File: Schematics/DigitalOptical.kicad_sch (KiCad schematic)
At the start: 112 parts, among them Q1 BSS138, Q2 BSS138, Q3 BSS138, Q4 BSS138, Q5 BSS138, Q6 BSS138, U100 PC817, U63 PC817, U64 PC817, U65 PCF8575, U66 PC817, U67 PC817, U68 PC817, U69 PC817, U70 PC817, U71 PC817, U72 PC817, U73 PC817, U74 LM1117-3.3, U75 PC817, U76 PC817, U77 PCF8575, U78 PCF8575, U79 PC817, U80 PC817, U81 PC817, U82 PC817, U83 PC817, U84 PC817, U85 PC817, U86 PC817, U87 LM1117-3.3, U88 LM1117-3.3, U89 PC817, U90 PC817, U91 PC817, U92 PC817, U93 PC817, U94 PC817, U95 PC817, U96 PC817, U97 PC817, U98 PC817, U99 PC817

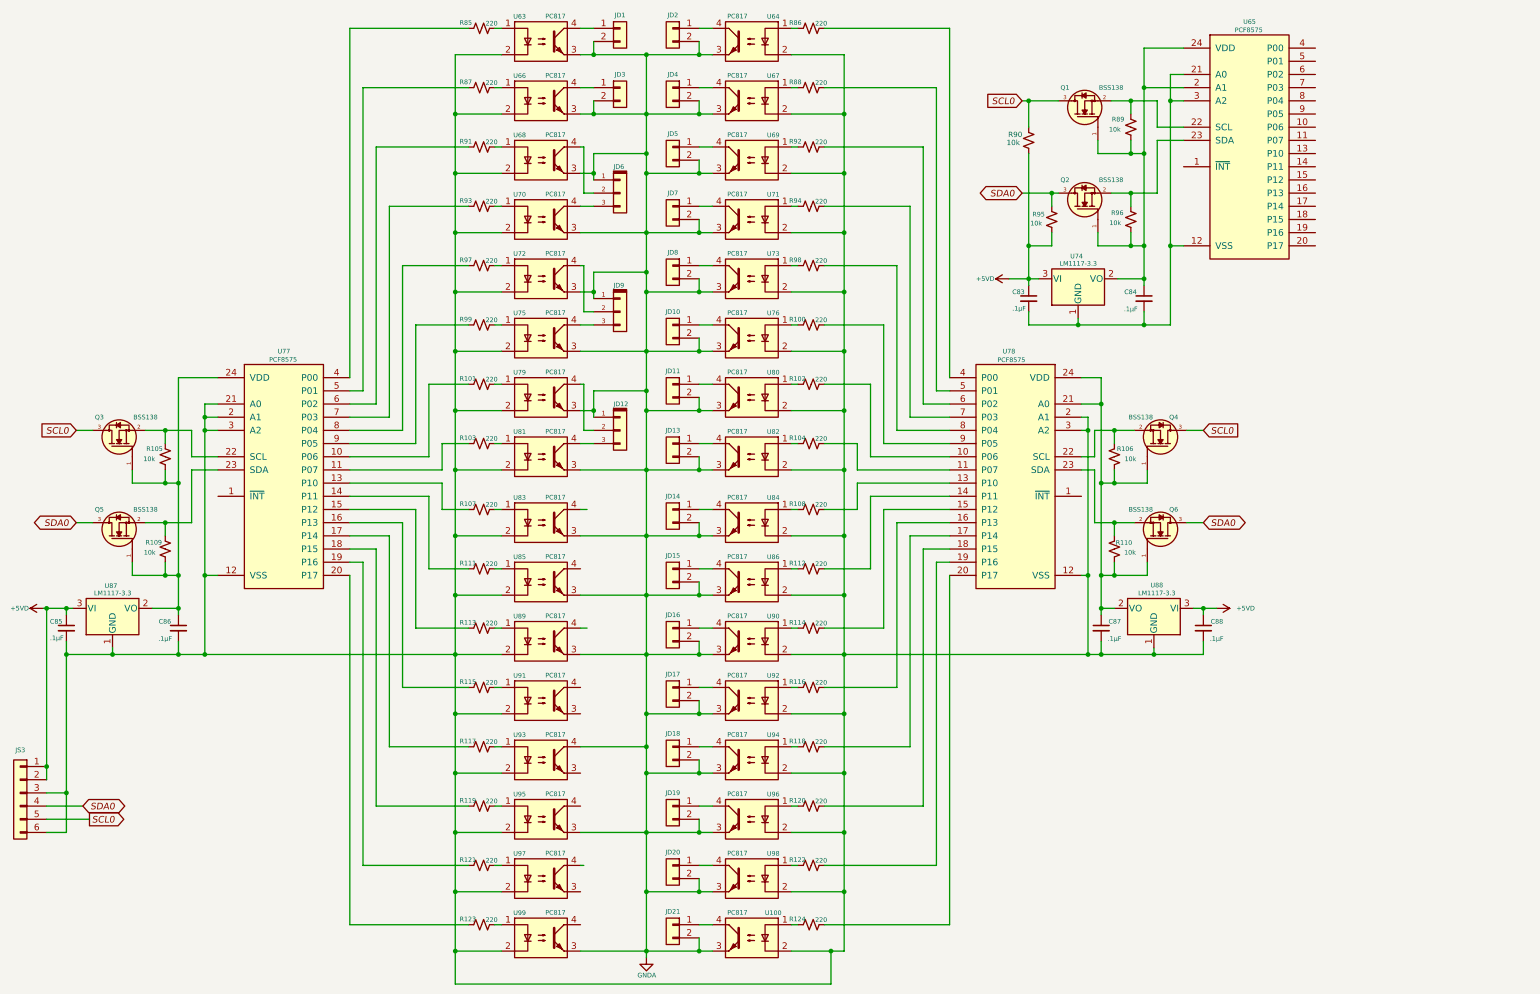
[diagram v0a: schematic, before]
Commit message: Prelude to split configurations.
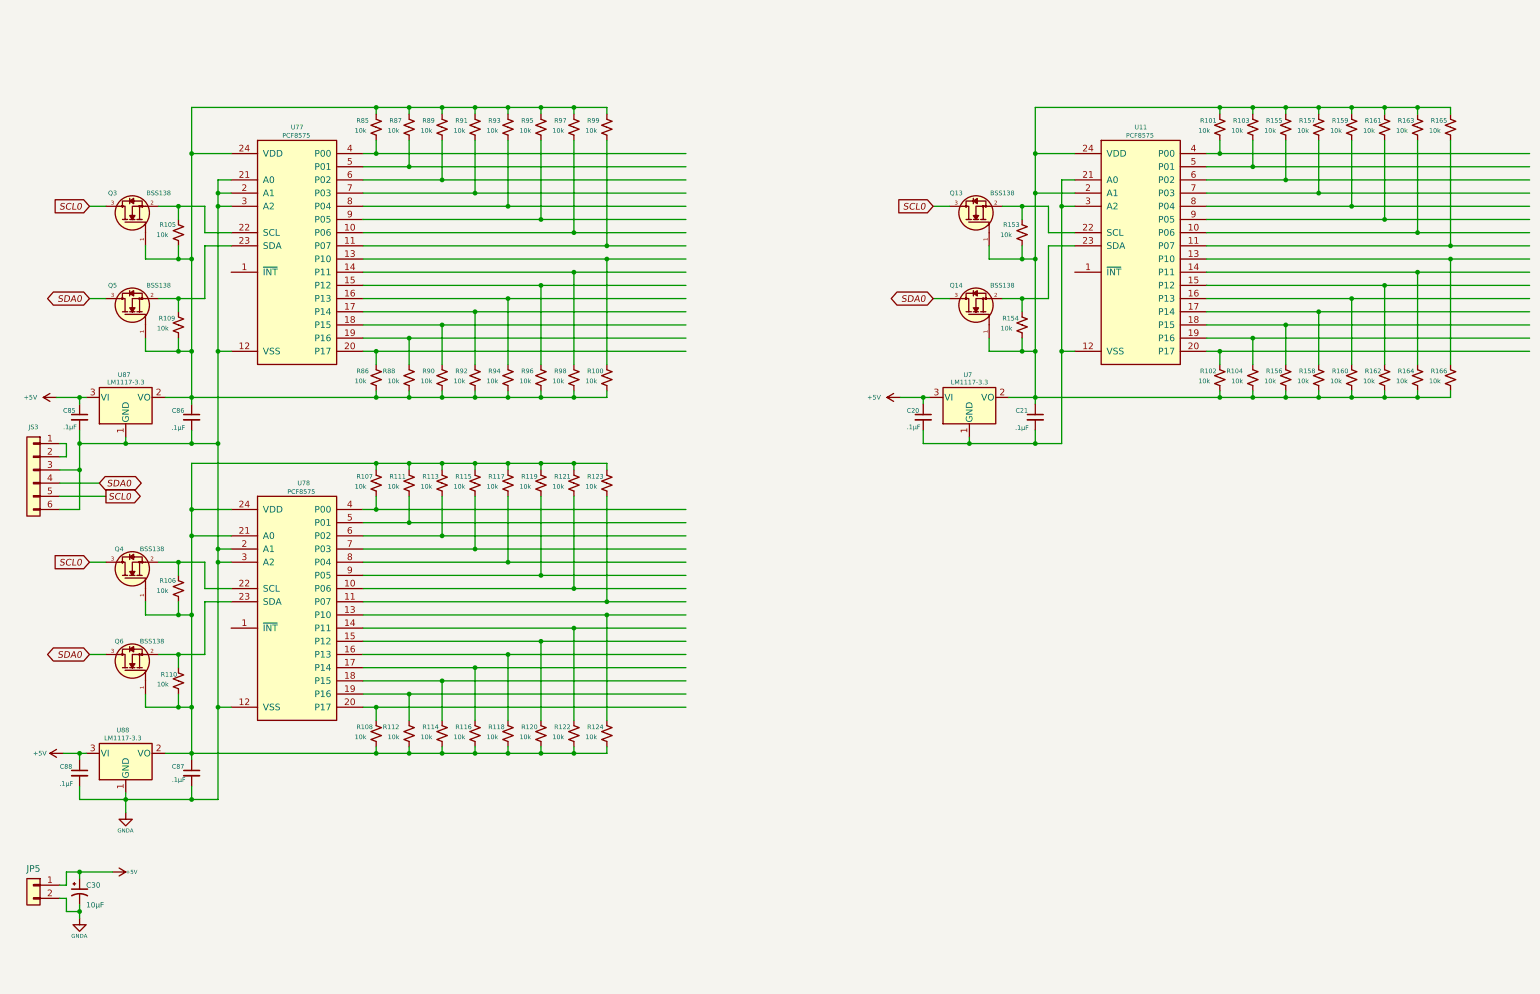
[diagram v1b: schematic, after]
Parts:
- removed C83, C84: .1µF, symbol Device:C_Small
- removed JD1, JD10, JD11, JD13, JD14, JD15, JD16, JD17, JD18, JD19, JD2, JD20, JD21, JD3, JD4, JD5, JD7, JD8: From 12v Analog, symbol Connector_Generic:Conn_01x02
- removed JD12, JD6, JD9: Conn_01x03, symbol Connector_keyed_kicad_sym:Conn_01x03
- removed Q1, Q2: BSS138, digikey-footprints:SOT-23-3, symbol dk_Transistors-FETs-MOSFETs-Single:BSS138
- removed U100, U63, U64, U66, U67, U68, U69, U70, U71, U72, U73, U75, U76, U79, U80, U81, U82, U83, U84, U85, U86, U89, U90, U91, U92, U93, U94, U95, U96, U97, U98, U99: PC817, Package_DIP:DIP-4_W7.62mm, symbol Isolator:PC817
- removed U65: PCF8575, IPC7351-Nominal:SOP65P775X200-24, symbol NXP:PCF8575
- removed U74: LM1117-3.3, symbol Regulator_Linear:LM1117-3.3
- added C20, C21: .1µF, symbol Device:C_Small
- added C30: 10µF, symbol Device:C_Polarized_Small_US
- added JP5: From 12v Analog, symbol Connector_Generic:Conn_01x02
- added Q13, Q14: BSS138, digikey-footprints:SOT-23-3, symbol dk_Transistors-FETs-MOSFETs-Single:BSS138
- added R153, R154, R155, R156, R157, R158, R159, R160, R161, R162, R163, R164, R165, R166: 10k, symbol Device:R_Small_US
- added U11: PCF8575, IPC7351-Nominal:SOP65P775X200-24, symbol NXP:PCF8575
- added U7: LM1117-3.3, symbol Regulator_Linear:LM1117-3.3
- R100, R101, R102, R103, R104, R107, R108, R111, R112, R113, R114, R115, R116, R117, R118, R119, R120, R121, R122, R123, R124, R85, R86, R87, R88, R91, R92, R93, R94, R97, R98, R99: value 220 -> 10k
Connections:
- net GNDA: now also C85.2, C86.2, C87.2, C88.2, JS3.3 (Pin_3), JS3.6 (Pin_6), U77.12 (VSS), U77.2 (A1), U77.21 (A0), U77.3 (A2), U78.12 (VSS), U78.2 (A1), U78.3 (A2), U87.1 (GND), U88.1 (GND), C30.2, JP5.2 (Pin_2)
- net SCL0: now also Q13.3; no longer R90.1
- net SDA0: now also Q14.3; no longer R95.1
- net at R120.2: now also C87.1, Q4.1, Q6.1, R106.2, R107.1, R108.2, R110.2, R111.1, R112.2, R113.1, R114.2, R115.1, R116.2, R117.1, R118.2, R119.1, R121.1, R122.2, R123.1, R124.2, U78.21 (A0), U78.24 (VDD), U88.2 (VO)
- net at R86.2: now also C86.1, Q3.1, Q5.1, R100.2, R105.2, R109.2, R85.1, R87.1, R88.2, R89.1, R90.2, R91.1, R92.2, R93.1, R94.2, R95.1, R96.2, R97.1, R98.2, R99.1, U77.24 (VDD), U87.2 (VO)
- net at R118.1: now also U78.16 (P13); no longer U78.17 (P14)
- net at U77.18 (P15): now also R90.1; no longer R119.2
- net at U77.9 (P05): now also R95.2; no longer R99.2
- net at R120.1: now also U78.15 (P12); no longer U78.18 (P15)
- net at R101.1: now also R102.2, R103.1, R104.2, C21.1, Q13.1, Q14.1, R153.2, R154.2, R155.1, R156.2, R157.1, R158.2, R159.1, R160.2, R161.1, R162.2, R163.1, R164.2, R165.1, R166.2, U11.2 (A1), U11.24 (VDD), U7.2 (VO)
- net at U78.10 (P06): now also R121.2; no longer R102.1
- net at R114.1: now also U78.18 (P15); no longer U78.15 (P12)
- net at U78.11 (P07): now also R123.2; no longer R104.1
- net at U78.9 (P05): now also R119.2; no longer R100.1
- net at U78.5 (P01): now also R111.2; no longer R88.1
- net at U77.14 (P11): now also R98.1; no longer R111.2
- net at R97.2: now also U77.10 (P06); no longer U77.8 (P04)
- net at R89.2: now also U77.6 (P02); no longer R96.2
- net at R96.1: now also U77.15 (P12)
- net at R113.2: now also U78.6 (P02); no longer U77.15 (P12)
- net at R107.2: now also U78.4 (P00); no longer U77.13 (P10)
- net at U77.7 (P03): now also R91.2; no longer R93.2
- net at R124.1: now also U78.13 (P10); no longer U78.20 (P17)
- net at R122.1: now also U78.14 (P11); no longer U78.19 (P16)
- net at R92.1: now also U77.17 (P14); no longer U78.6 (P02)
- net at R103.2: now also U11.5 (P01); no longer U77.11 (P07)
- net at R108.1: now also U78.20 (P17); no longer U78.13 (P10)
- net at R101.2: now also U11.4 (P00); no longer U77.10 (P06)
- net at U77.16 (P13): now also R94.1; no longer R115.2
- net at R117.2: now also U78.8 (P04); no longer U77.17 (P14)
- net at U77.19 (P16): now also R88.1; no longer R121.2
- net at U77.20 (P17): now also R86.1; no longer R123.2
- net at R112.1: now also U78.19 (P16); no longer U78.14 (P11)
- net at R116.1: now also U78.17 (P14); no longer U78.16 (P13)
- net at U78.7 (P03): now also R115.2; no longer R94.1
- net +5VD renamed +5V
- net +5V: now also C20.1, C30.1, JP5.1 (Pin_1), U7.3 (VI); no longer JS3.1 (Pin_1), JS3.2 (Pin_2), R90.2, R95.2
- new net: C20.2, C21.2, U11.12 (VSS), U11.21 (A0), U11.3 (A2), U7.1 (GND)
- new net: R157.2, U11.7 (P03)
- new net: R155.2, U11.6 (P02)
- new net: R164.1, U11.14 (P11)
- new net: Q14.2, R154.1, U11.23 (SDA)
- new net: R100.1, U77.13 (P10)
- new net: R159.2, U11.8 (P04)
- new net: R163.2, U11.10 (P06)
- new net: R165.2, U11.11 (P07)
- new net: R99.2, U77.11 (P07)
- new net: R93.2, U77.8 (P04)
- new net: Q13.2, R153.1, U11.22 (SCL)
- new net: R104.1, U11.19 (P16)
- new net: R162.1, U11.15 (P12)
- new net: R166.1, U11.13 (P10)
- new net: JS3.1 (Pin_1), JS3.2 (Pin_2)
- new net: R156.1, U11.18 (P15)
- new net: R161.2, U11.9 (P05)
- new net: R158.1, U11.17 (P14)
- new net: R160.1, U11.16 (P13)
- new net: R102.1, U11.20 (P17)
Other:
- moved on the sheet: C85, C86, C87, C88, JS3, Q3, Q4, Q5, Q6, R105, R106, R109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
